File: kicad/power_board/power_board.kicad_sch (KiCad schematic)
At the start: 94 parts, among them IC1 LTC4151IMS-1#PBF, J1 24V, J10 Grid, J11 GRID_CTRL, J12 MCU_2, J14 5V, J15 MCU_P_RES, J16 MCU_BTN1, J17 MCU_BTN2, J18 BTN1, J19 BTN2, J2 24V, J20 MCU_GND, J21 SOLAR_CTRL, J22 CTRL, J3 GND, J4 GND, J5 GND, J6 GND, J7 MCU, J9 Solar Panel, Q1 FDD8453LZ, Q10 MOCD207M, Q2 FDD8453LZ, Q3 FDD8453LZ, Q4 FDD8453LZ, Q5 FDS5670, Q6 MOCD207M, Q7 MOCD207M, Q8 FDD8453LZ, Q9 MOCD207M, U5 LT3757A, U6 LT1161

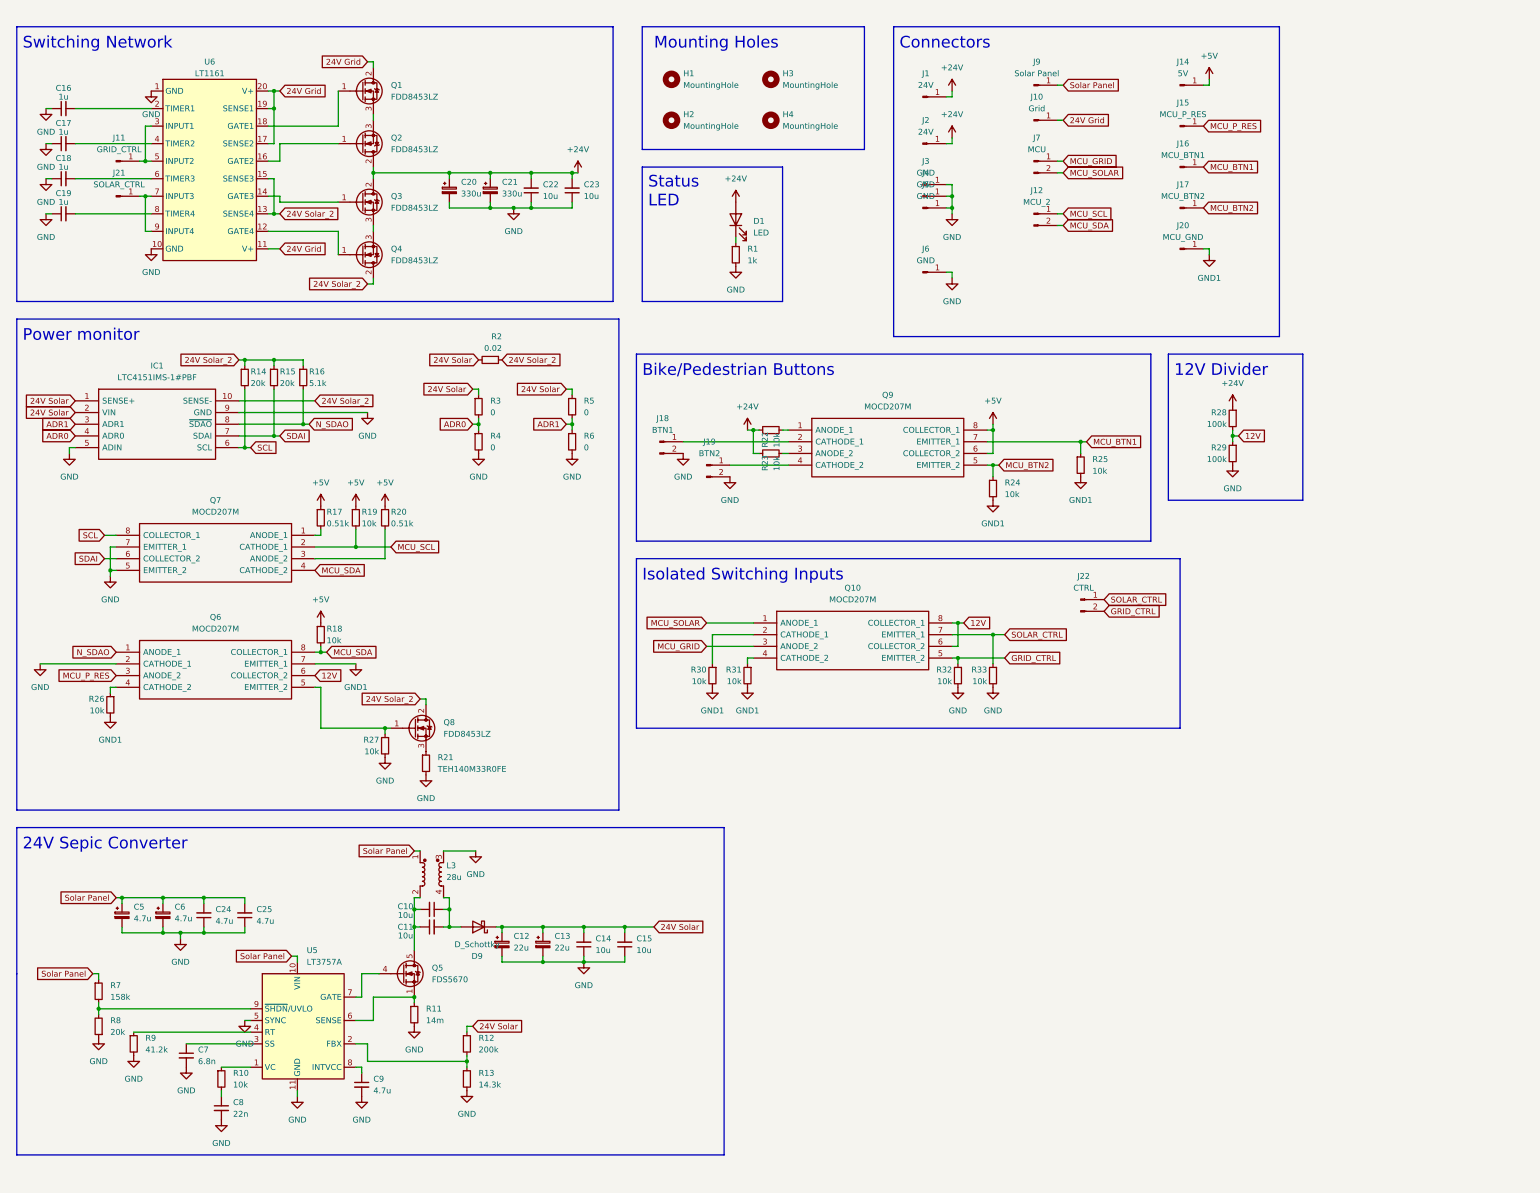
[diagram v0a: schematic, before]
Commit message: update pcbs
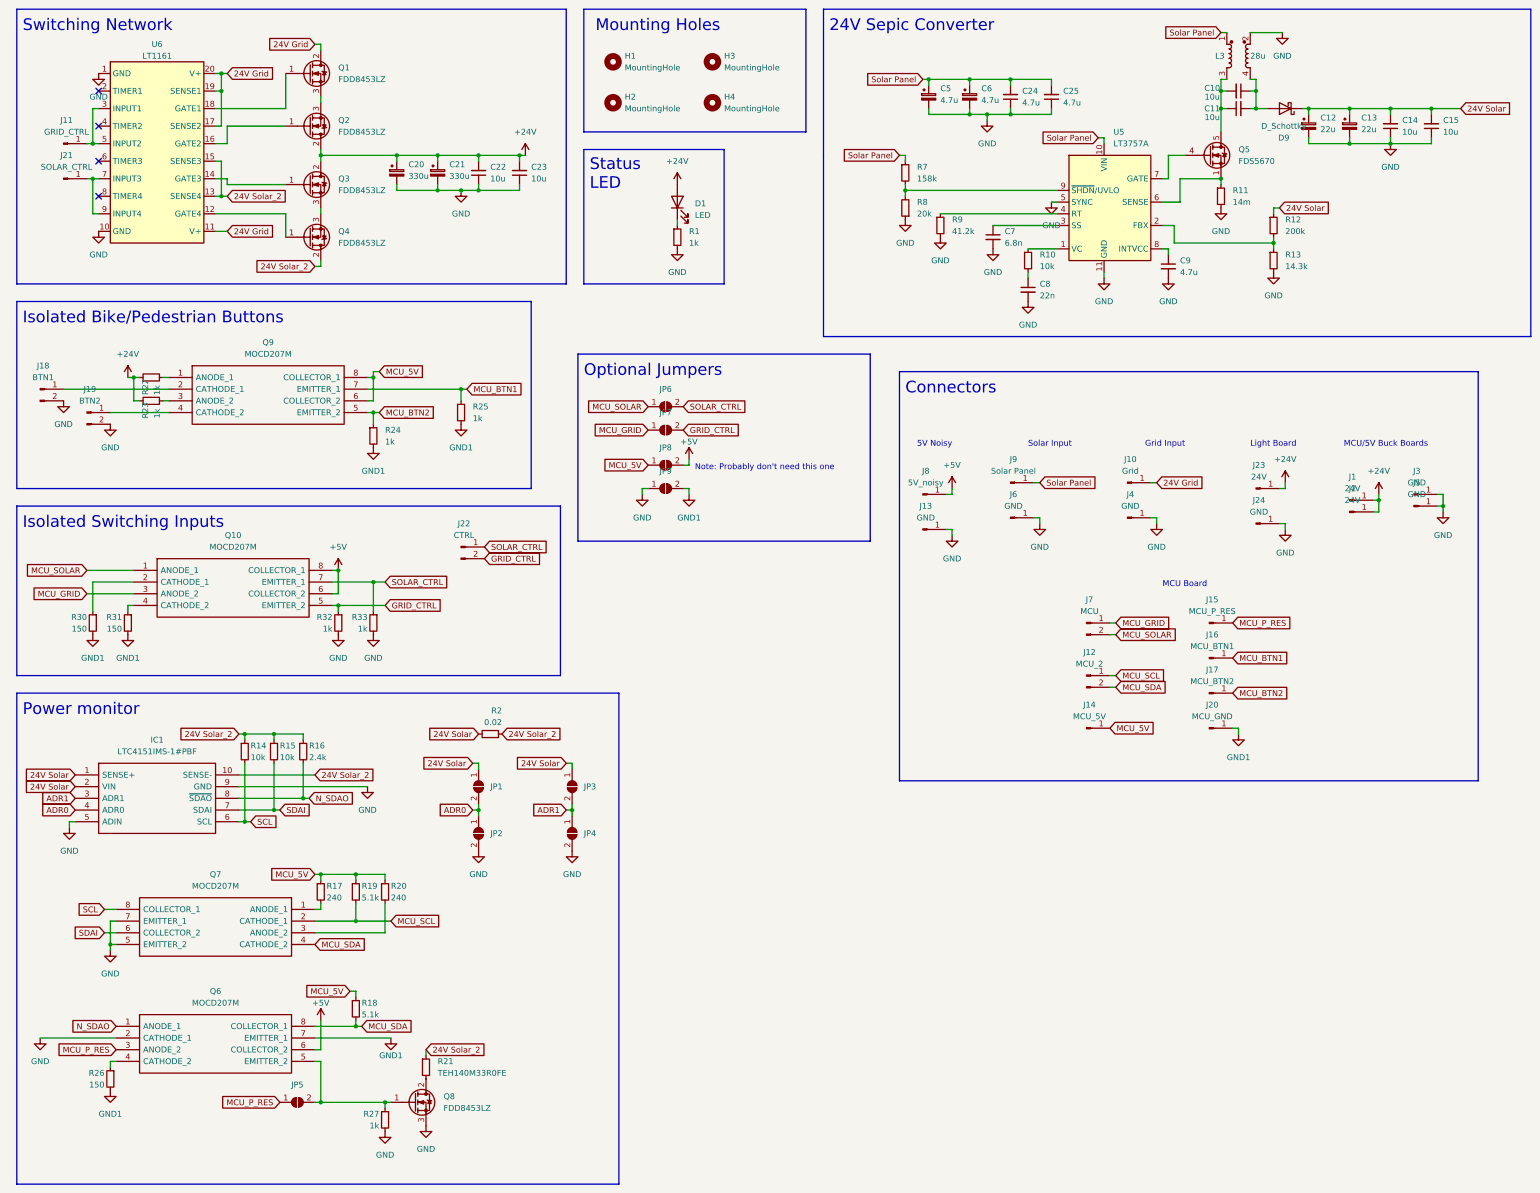
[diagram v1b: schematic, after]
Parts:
- removed C16, C17, C18, C19: 1u, Capacitor_SMD:C_0603_1608Metric, symbol Device:C_Small
- removed R28, R29: 100k, Resistor_SMD:R_1206_3216Metric, symbol Device:R_Small
- removed R3, R4, R5, R6: 0, Resistor_SMD:R_2512_6332Metric, symbol Device:R_Small
- added J13: GND, Connector_PinHeader_2.54mm:PinHeader_1x01_P2.54mm_Vertical, symbol Connector:Conn_01x01_Male
- added J23: 24V, _mylib:hole, symbol Connector:Conn_01x01_Male
- added J24: GND, _mylib:hole, symbol Connector:Conn_01x01_Male
- added J8: 5V_noisy, Connector_PinHeader_2.54mm:PinHeader_1x01_P2.54mm_Vertical, symbol Connector:Conn_01x01_Male
- added JP1, JP2, JP3, JP4, JP5, JP6, JP7, JP8, JP9: SolderJumper_2_Open, Jumper:SolderJumper-2_P1.3mm_Open_TrianglePad1.0x1.5mm, symbol Jumper:SolderJumper_2_Open
- C24, C25: footprint Capacitor_SMD:C_1210_3225Metric -> Capacitor_SMD:C_0805_2012Metric
- J10, J4: footprint Connector_PinHeader_2.54mm:PinHeader_1x01_P2.54mm_Vertical -> _mylib:hole
- J14: value 5V -> MCU_5V
- J6, J9: footprint _mine:73099 -> _mylib:hole_1.6mm
- Q5: footprint Package_TO_SOT_SMD:LFPAK33 -> Package_SO:SOIC-8_3.9x4.9mm_P1.27mm
- R1: footprint Resistor_SMD:R_2512_6332Metric -> Resistor_SMD:R_0603_1608Metric
- R14, R15: value 20k -> 10k
- R16: value 5.1k -> 2.4k
- R17, R20: value 0.51k -> 240; footprint Resistor_SMD:R_0805_2012Metric -> Resistor_SMD:R_0603_1608Metric
- R18, R19: value 10k -> 5.1k; footprint Resistor_SMD:R_0805_2012Metric -> Resistor_SMD:R_0603_1608Metric
- R21: footprint Resistor_THT:R_Axial_DIN0207_L6.3mm_D2.5mm_P10.16mm_Horizontal -> _mylib:TEH140
- R22, R23, R24, R25, R27, R32, R33: value 10k -> 1k; footprint Resistor_SMD:R_0805_2012Metric -> Resistor_SMD:R_0603_1608Metric
- R26, R30, R31: value 10k -> 150; footprint Resistor_SMD:R_0805_2012Metric -> Resistor_SMD:R_0603_1608Metric
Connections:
- net 12V is gone; now on net +5V: Q10.6 (COLLECTOR_2), Q10.8 (COLLECTOR_1), Q6.6 (COLLECTOR_2)
- net +24V: now also J23.1 (Pin_1)
- net +5V: now also J8.1 (Pin_1), JP8.2 (B); no longer J14.1 (Pin_1), Q9.6 (COLLECTOR_2), Q9.8 (COLLECTOR_1), R17.1, R18.1, R19.1, R20.1
- net 24V Solar: now also JP1.1 (A), JP3.1 (A)
- net 24V Solar_2: now also R21.1; no longer Q8.2 (D)
- net ADR0: now also JP1.2 (B), JP2.1 (A)
- net ADR1: now also JP3.2 (B), JP4.1 (A)
- net GND: now also L3.2, Q8.3 (S), J13.1 (Pin_1), J24.1 (Pin_1), JP2.2 (B), JP4.2 (B), JP9.1 (A); no longer L3.3, R21.2
- net GND1: now also JP9.2 (B)
- net GRID_CTRL: now also JP7.2 (B)
- net MCU_GRID: now also JP7.1 (A)
- net MCU_P_RES: now also JP5.1 (A)
- net MCU_SOLAR: now also JP6.1 (A)
- net SOLAR_CTRL: now also JP6.2 (B)
- net at Q6.5 (EMITTER_2), Q8.1 (G), R27.1: now also JP5.2 (B)
- net at C10.2, C11.1, Q5.5 (D): now also L3.3, Q5.6 (S), Q5.7 (S), Q5.8 (S); no longer L3.2
- new net: Q8.2 (D), R21.2
- new net MCU_5V: J14.1 (Pin_1), JP8.1 (A), Q9.6 (COLLECTOR_2), Q9.8 (COLLECTOR_1), R17.1, R18.1, R19.1, R20.1
- no-connect marks 0 -> 4
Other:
- note added: "5V Noisy"
- note added: "Grid Input"
- note added: "Isolated Bike/Pedestrian Buttons"
- note added: "Light Board"
- note added: "MCU Board"
- note added: "MCU/5V Buck Boards"
- note added: "Note: Probably don't need this one"
- note added: "Optional Jumpers"
- note added: "Solar Input"
- note removed: "12V Divider"
- note removed: "Bike/Pedestrian Buttons"
- moved on the sheet: C10, C11, C12, C13, C14, C15, C20, C21, C22, C23, C24, C25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
